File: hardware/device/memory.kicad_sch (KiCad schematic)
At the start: 9 parts, among them IC2 IS42S16160J-7BLI, J3 MICRO_SD

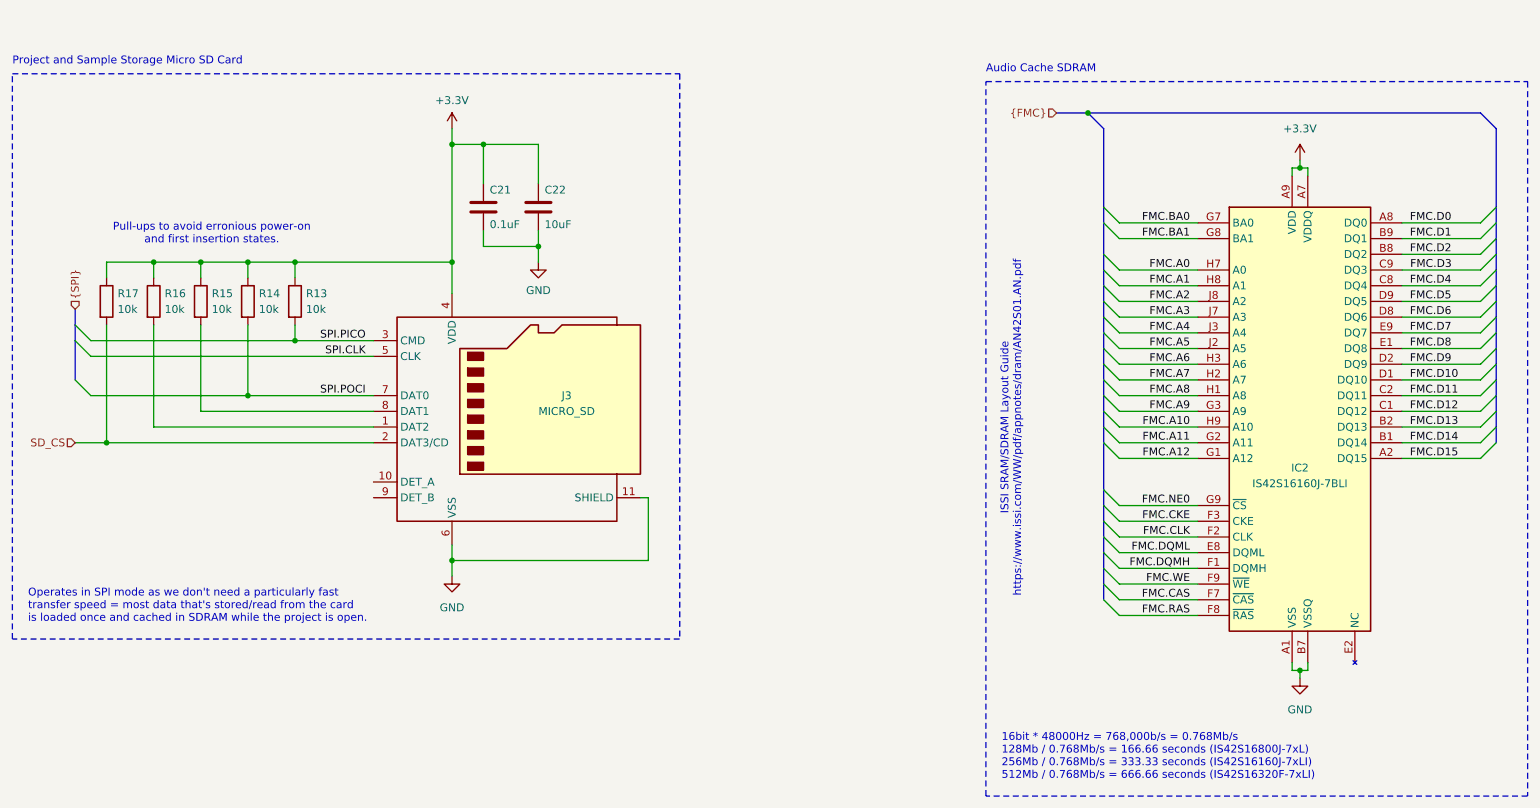
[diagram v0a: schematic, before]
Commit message: feat: various audio and power schematic layout
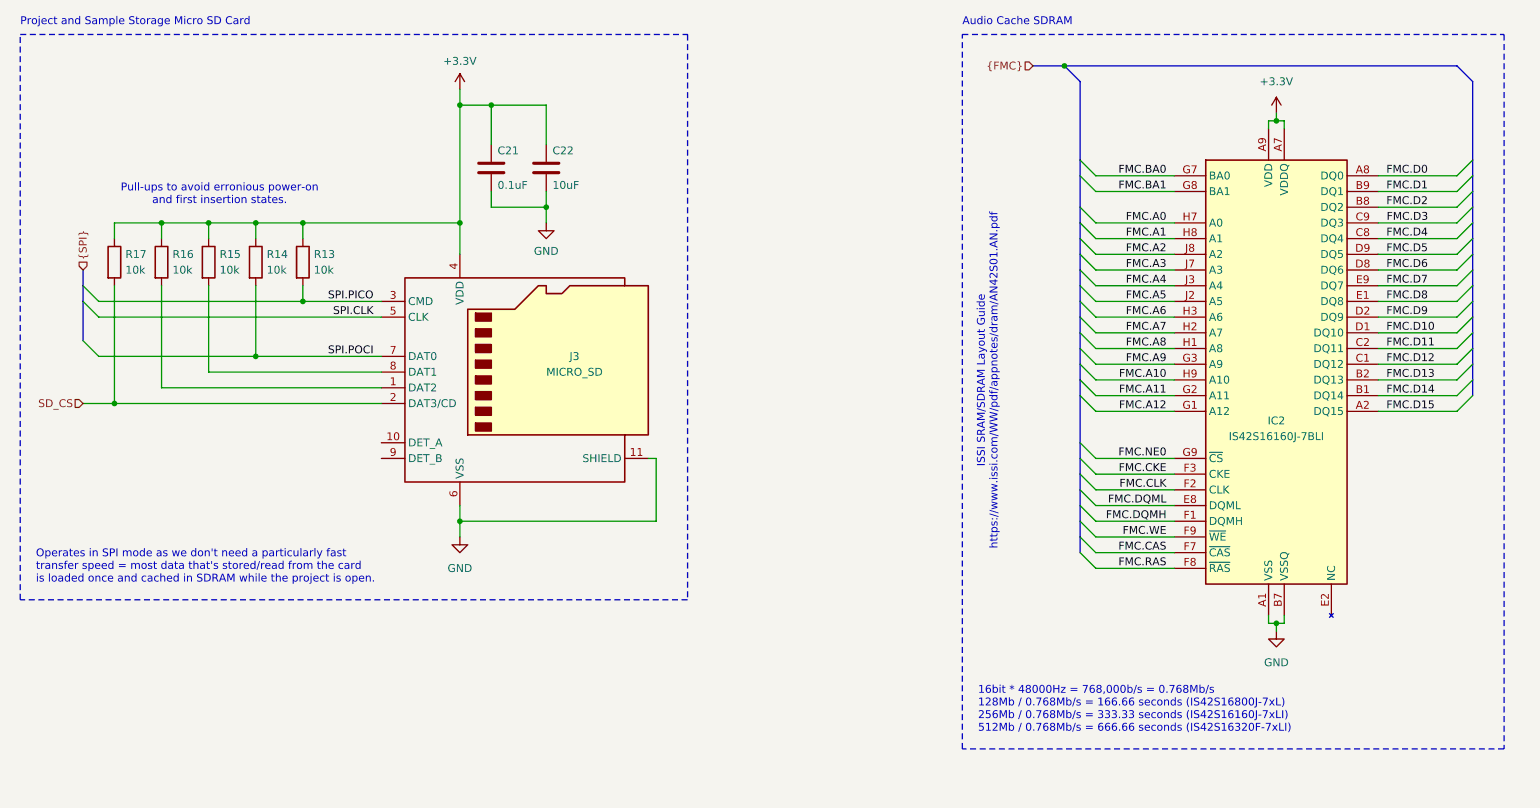
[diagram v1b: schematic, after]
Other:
- moved on the sheet: C21, C22, IC2, J3, R13, R14, R15, R16, R17
